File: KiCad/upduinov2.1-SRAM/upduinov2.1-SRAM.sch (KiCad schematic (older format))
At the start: 4 parts, among them J1 Conn_01x16_Male, J2 Conn_01x18_Male, U1 CY62157

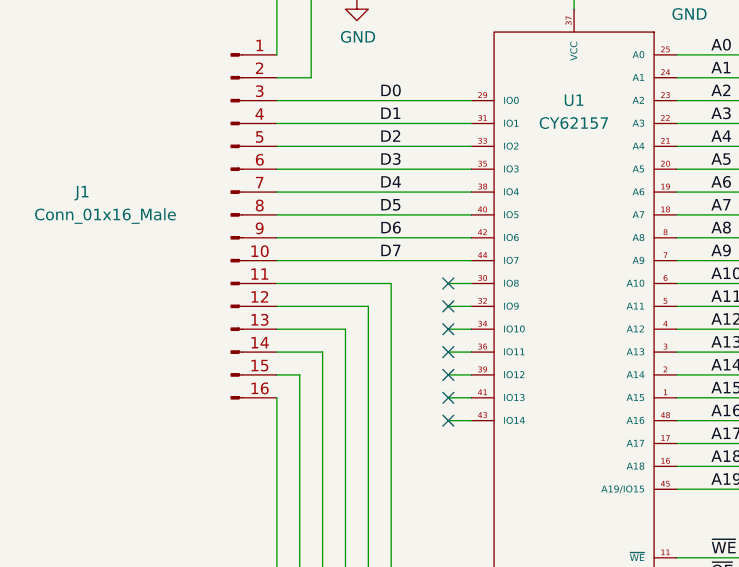
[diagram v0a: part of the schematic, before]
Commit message: updv2 pcb v1 w handroute decoupler
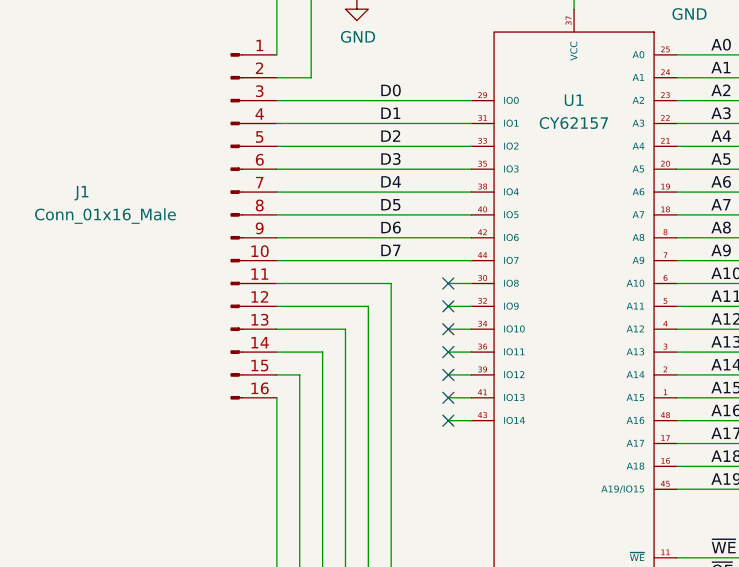
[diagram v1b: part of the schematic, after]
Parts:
- J1: footprint (none) -> Connector_PinHeader_2.54mm:PinHeader_1x16_P2.54mm_Vertical
- J2: footprint (none) -> Connector_PinHeader_2.54mm:PinHeader_1x18_P2.54mm_Vertical
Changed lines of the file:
@@
 $EndComp
 $Comp
-L power:GND #PWR?
+L power:GND #PWR0101
 U 1 1 5DEF48CC
 P 5750 1800
-F 0 "#PWR?" H 5750 1550 50  0001 C CNN
+F 0 "#PWR0101" H 5750 1550 50  0001 C CNN
 F 1 "GND" H 5755 1627 50  0000 C CNN
 F 2 "" H 5750 1800 50  0001 C CNN
@@
 $EndComp
 $Comp
-L power:+3.3V #PWR?
+L power:+3.3V #PWR0102
 U 1 1 5DEF4D9D
 P 5250 1750
-F 0 "#PWR?" H 5250 1600 50  0001 C CNN
+F 0 "#PWR0102" H 5250 1600 50  0001 C CNN
 F 1 "+3.3V" H 5265 1923 50  0000 C CNN
 F 2 "" H 5250 1750 50  0001 C CNN
@@
 $EndComp
 $Comp
-L power:GND #PWR?
+L power:GND #PWR0103
 U 1 1 5DEF64C9
 P 5250 5350
-F 0 "#PWR?" H 5250 5100 50  0001 C CNN
+F 0 "#PWR0103" H 5250 5100 50  0001 C CNN
 F 1 "GND" H 5100 5250 50  0000 C CNN
 F 2 "" H 5250 5350 50  0001 C CNN
@@
 F 0 "J1" H 3100 2950 50  0000 C CNN
 F 1 "Conn_01x16_Male" H 3200 2850 50  0000 C CNN
-F 2 "" H 3750 2850 50  0001 C CNN
+F 2 "Connector_PinHeader_2.54mm:PinHeader_1x16_P2.54mm_Vertical" H 3750 2850 50  0001 C CNN
 F 3 "~" H 3750 2850 50  0001 C CNN
 	1    3750 2850
@@
 $EndComp
 $Comp
-L power:+3.3V #PWR?
+L power:+3.3V #PWR0104
 U 1 1 5DF23968
 P 6250 4600
-F 0 "#PWR?" H 6250 4450 50  0001 C CNN
+F 0 "#PWR0104" H 6250 4450 50  0001 C CNN
 F 1 "+3.3V" H 6100 4650 50  0000 C CNN
 F 2 "" H 6250 4600 50  0001 C CNN
@@
 F 0 "J2" H 6472 2724 50  0000 R CNN
 F 1 "Conn_01x18_Male" H 6472 2633 50  0000 R CNN
-F 2 "" H 6500 2750 50  0001 C CNN
+F 2 "Connector_PinHeader_2.54mm:PinHeader_1x18_P2.54mm_Vertical" H 6500 2750 50  0001 C CNN
 F 3 "~" H 6500 2750 50  0001 C CNN
 	1    6500 2750
@@
 	3950 1750 5250 1750
 $Comp
-L power:GND #PWR?
+L power:GND #PWR0105
 U 1 1 5DF8623F
 P 4300 1900
-F 0 "#PWR?" H 4300 1650 50  0001 C CNN
+F 0 "#PWR0105" H 4300 1650 50  0001 C CNN
 F 1 "GND" H 4305 1727 50  0000 C CNN
 F 2 "" H 4300 1900 50  0001 C CNN
@@
 Wire Wire Line
 	4450 5550 4450 3150
-Wire Wire Line
-	4450 3150 4400 3150
 NoConn ~ 4700 3150
 NoConn ~ 4700 3250
@@
 D7
 Wire Wire Line
-	4400 3150 3950 3150
+	3950 3150 4450 3150
 $EndSCHEMATC
